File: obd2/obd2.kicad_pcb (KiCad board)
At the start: 2 copper layers, 1 part, among them U2 385-MCP2551-I/SN

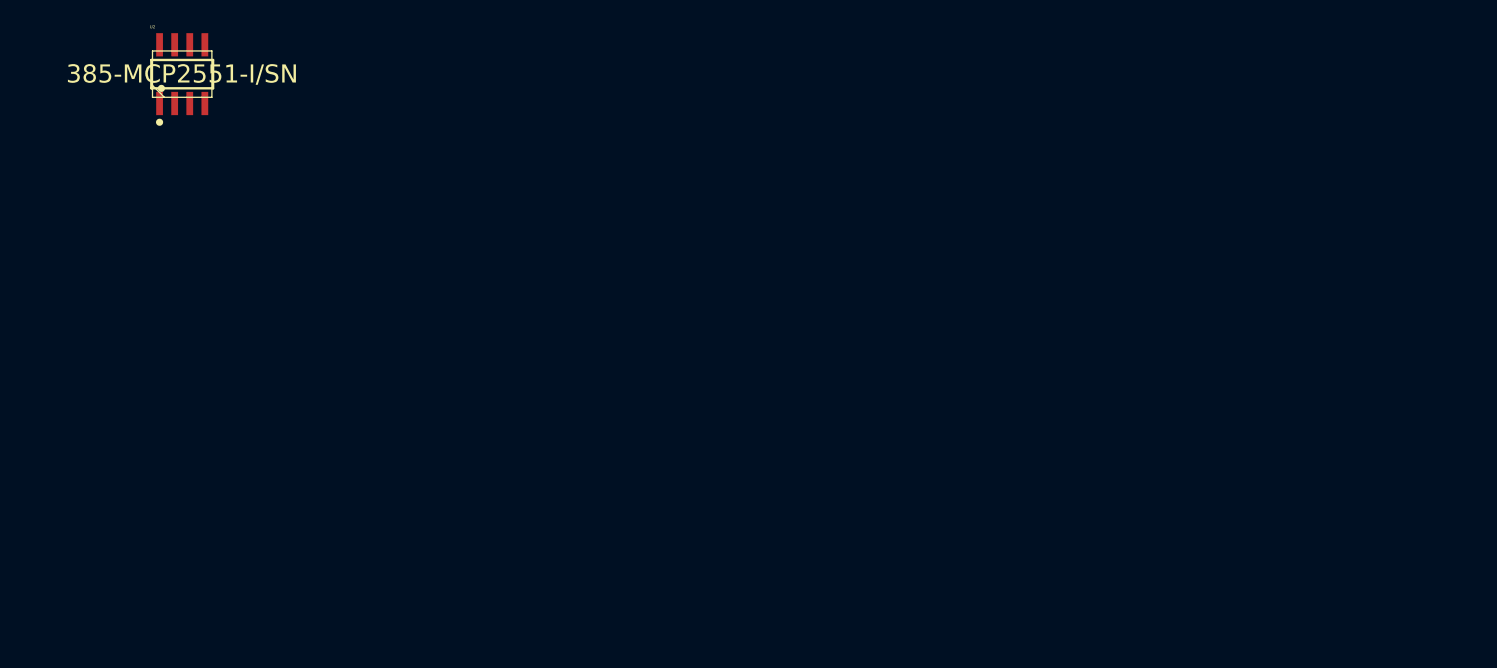
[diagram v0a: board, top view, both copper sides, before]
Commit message: Almost done schematic and component selections
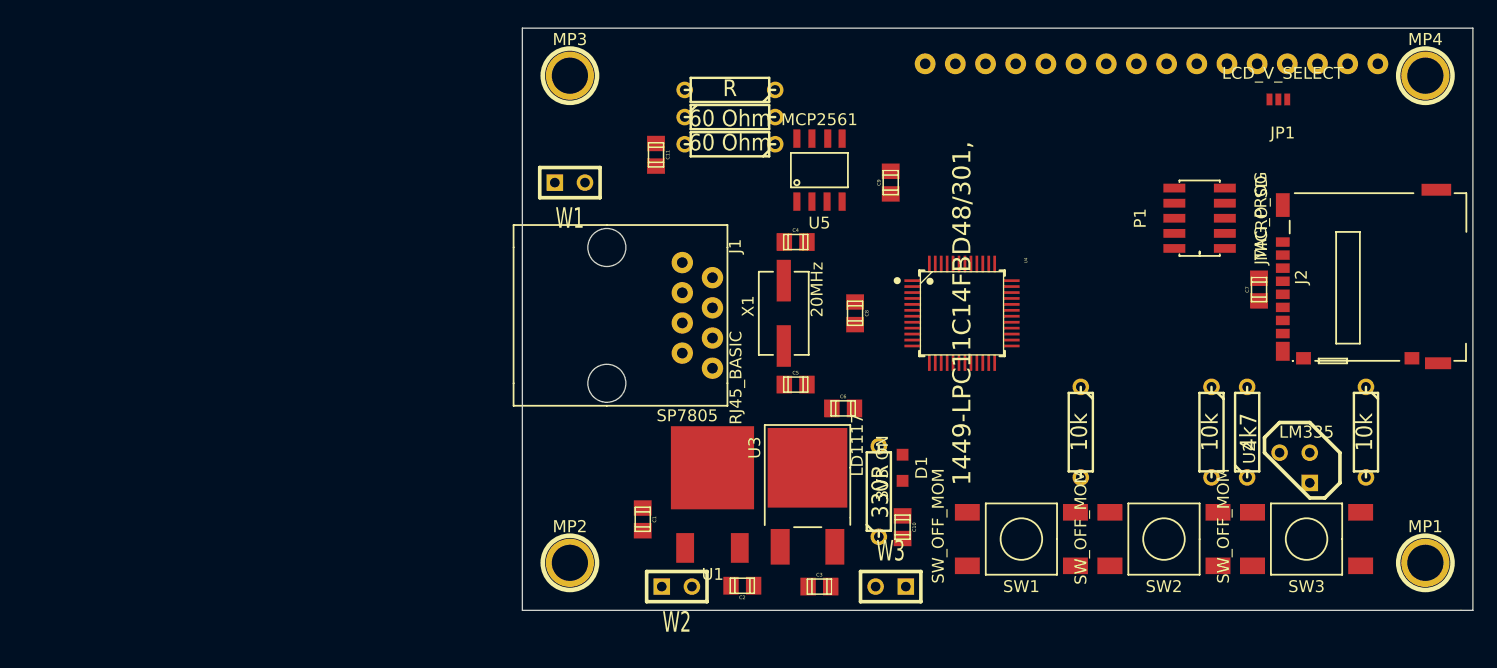
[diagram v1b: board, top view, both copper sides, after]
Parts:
- added C1: 0.33uF, c_0805, F.Cu at (205.1, 140.3)
- added C10: 0.1u, c_0805, F.Cu at (227.0, 141.0)
- added C11: C, c_0805, F.Cu at (206.2, 109.7)
- added C2: 0.1uF, c_0805, F.Cu at (213.5, 145.9)
- added C3: 0.1uF, c_0805, F.Cu at (220.0, 146.0)
- added C4: 39pF, c_0805, F.Cu at (218.0, 117.0)
- added C5: 39pF, c_0805, F.Cu at (218.0, 129.0)
- added C6: 10uF, c_0805, F.Cu at (222.0, 131.0)
- added C7: 0.1u, c_0805, F.Cu at (257.0, 121.0)
- added C8: 0.1u, c_0805, F.Cu at (223.0, 123.0)
- added C9: 0.1u, c_0805, F.Cu at (226.0, 112.0)
- added D1: 3V3_ON, LED_J_LEAD, F.Cu at (227.0, 136.0)
- added J1: RJ45_BASIC, RJ45, F.Cu at (211.0, 120.0)
- added J2: MICRO_SD, SD_502702_003, F.Cu at (259.0, 117.0)
- added JP1: LCD_V_SELECT, SOLDER_JUMPER_3, F.Cu at (259.0, 105.0)
- added LCD1: LCD16X2, GDM1602K, B.Cu at (267.0, 102.0)
- added MP1: SCREW_4-40, 1pin, F.Cu at (271.0, 144.0)
- added MP2: SCREW_4-40, 1pin, F.Cu at (199.0, 144.0)
- added MP3: SCREW_4-40, 1pin, F.Cu at (199.0, 103.0)
- added MP4: SCREW_4-40, 1pin, F.Cu at (271.0, 103.0)
- added P1: JTAG_PROG, GRPB052VWQS-RC, F.Cu at (252.0, 115.0)
- added R1: 330R, R3, F.Cu at (225.0, 138.0)
- added R2: R, R3, F.Cu at (212.5, 104.2)
- added R3: 60 Ohm, R3, F.Cu at (212.5, 108.8)
- added R4: 60 Ohm, R3, F.Cu at (212.5, 106.5)
- added R5: 4k7, R3, F.Cu at (256.0, 133.0)
- added R6: 10k, R3, F.Cu at (242.0, 133.0)
- added R7: 10k, R3, F.Cu at (253.0, 133.0)
- added R8: 10k, R3, F.Cu at (266.0, 133.0)
- added SW1: SW_OFF_MOM, FSM4JSMA_pushbutton, F.Cu at (237.0, 142.0)
- added SW2: SW_OFF_MOM, FSM4JSMA_pushbutton, F.Cu at (249.0, 142.0)
- added SW3: SW_OFF_MOM, FSM4JSMA_pushbutton, F.Cu at (261.0, 142.0)
- added U1: SP7805, TO-252-3, F.Cu at (211.0, 136.0)
- added U3: LD1117, DPAK, F.Cu at (219.0, 136.0)
- added U4: 1449-LPC11C14FBD48/301,, melissa/dintu, F.Cu at (232.0, 123.0)
- added U5: MCP2561, SOIC-8-Narrow, F.Cu at (220.0, 111.0)
- added W1: VBAT_T, SIL-2, F.Cu at (199.0, 112.0)
- added W2: 5V_T, SIL-2, F.Cu at (208.0, 146.0)
- added W3: 3V3_T, SIL-2, F.Cu at (226.0, 146.0)
- added X1: 20MHz, CSM-3X, F.Cu at (217.0, 123.0)
- U2: value 385-MCP2551-I/SN -> LM335; footprint Plecharts/b6cyy -> TO92
- moved U2 99.3 mm to (260.0, 136.0), turned to 270 degrees
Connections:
- U2 pad 1: (no net) -> GND
- U2 pad 2: (no net) -> TEMP
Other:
- board outline added: 80 x 49 mm
